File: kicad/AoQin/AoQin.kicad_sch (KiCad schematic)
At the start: 12 parts, among them J1 Conn_02x03_Odd_Even, J10 1869237, J3 1869237, J4 1869237, J5 1869237, J6 1869237, J7 1869237, J8 Screw_Terminal_01x03, J9 Screw_Terminal_01x03

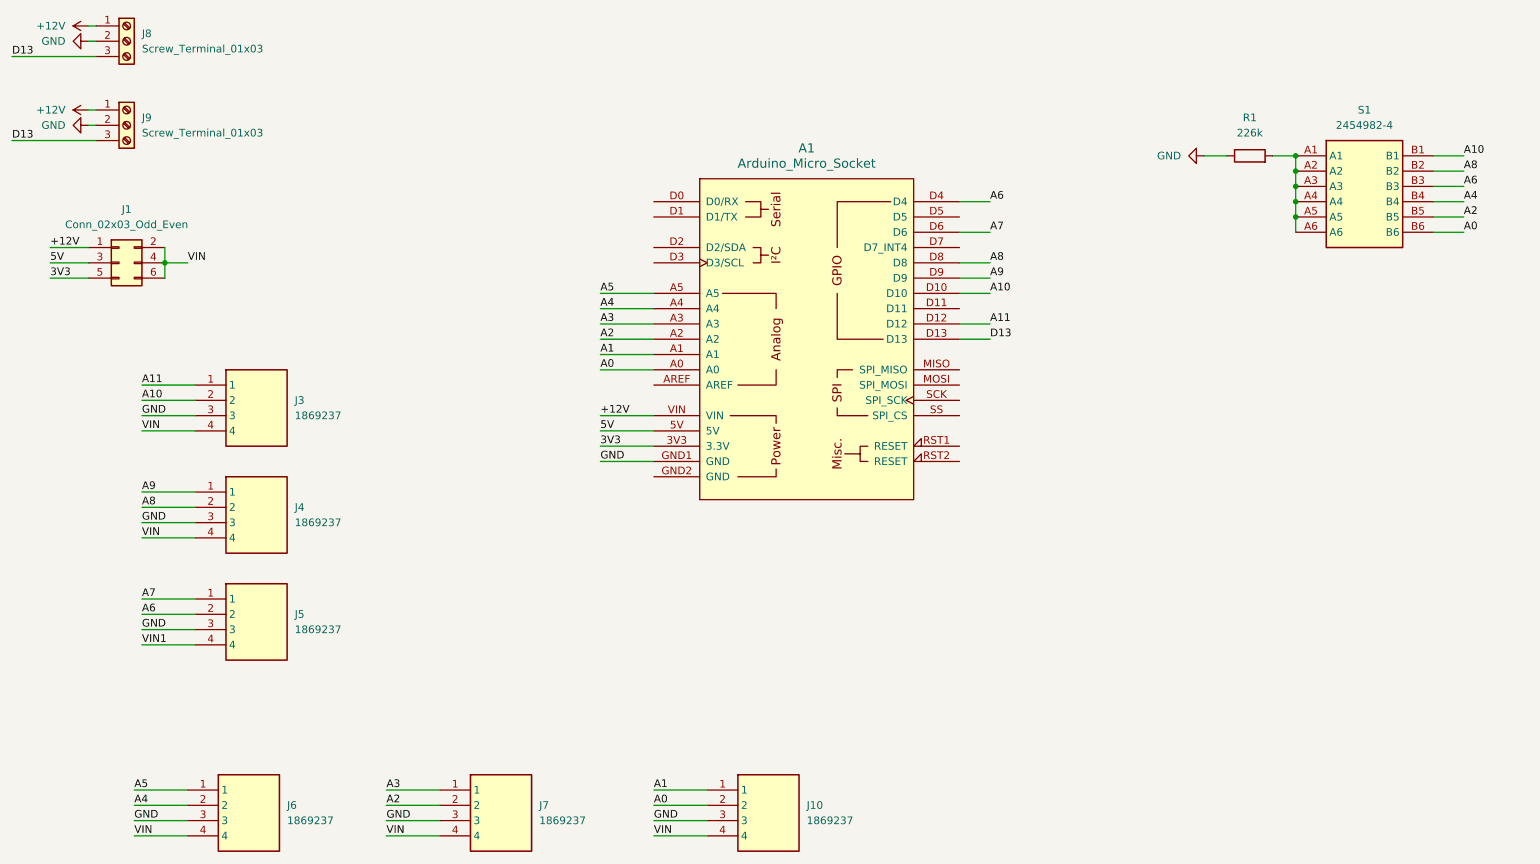
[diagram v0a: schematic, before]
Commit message: If I Had a Hammer
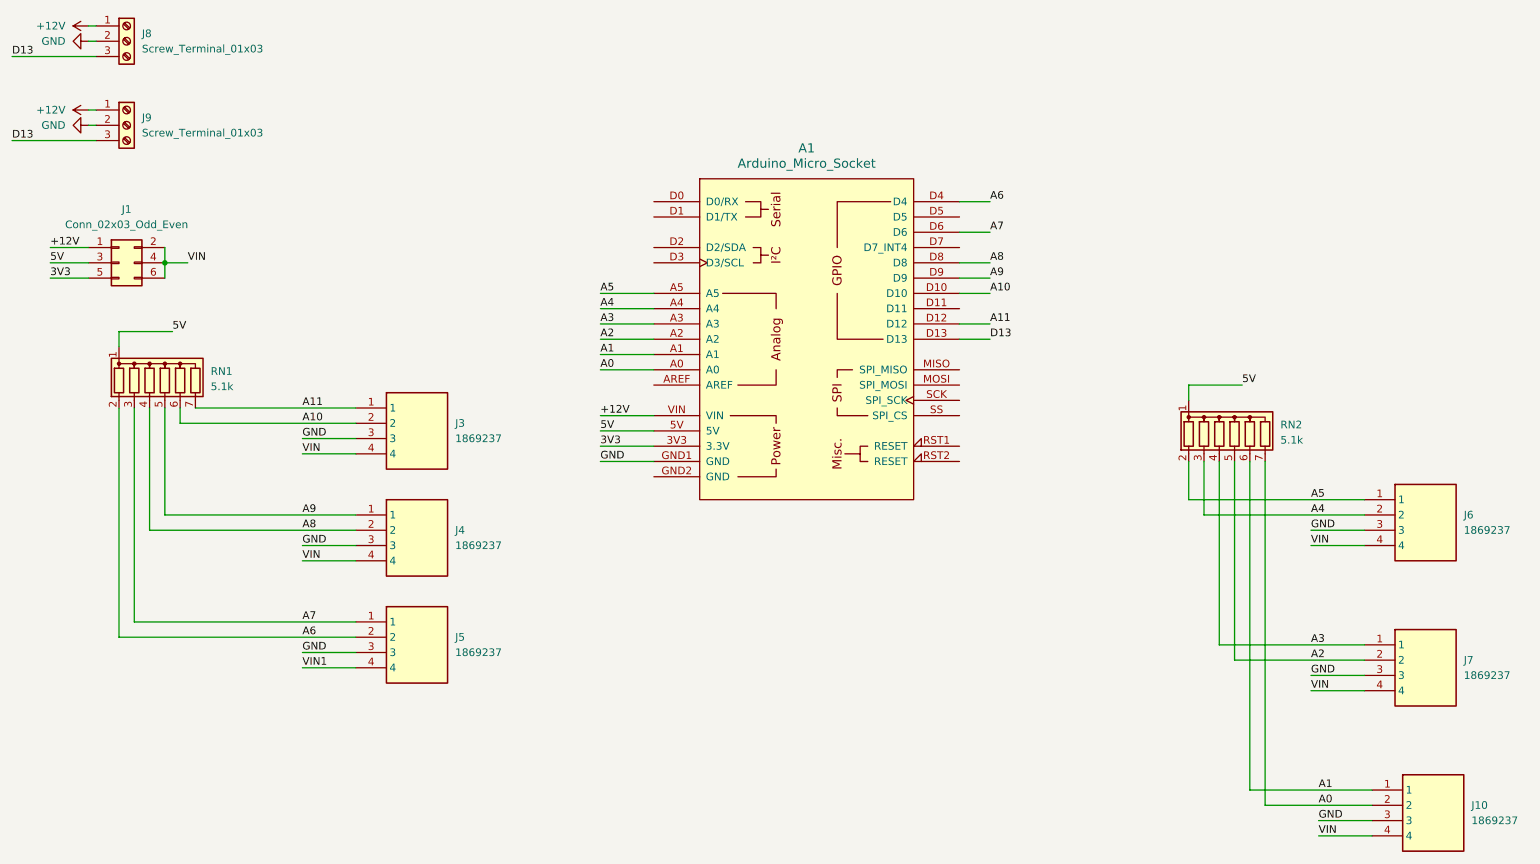
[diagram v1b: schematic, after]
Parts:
- removed R1: 226k, Resistor_THT:R_Axial_DIN0207_L6.3mm_D2.5mm_P7.62mm_Horizontal, symbol Device:R
- removed S1: 2454982-4, footprints:24549824, symbol 2454982-4:2454982-4
- added RN1, RN2: 5.1k, Resistor_THT:R_Array_SIP7, symbol Device:R_Network06
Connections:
- net 5V: now also RN1.1 (common), RN2.1 (common)
- net A0: now also RN2.7 (R6)
- net A1: now also RN2.6 (R5)
- net A10: now also RN1.6 (R5)
- net A11: now also RN1.7 (R6)
- net A2: now also RN2.5 (R4)
- net A3: now also RN2.4 (R3)
- net A4: now also RN2.3 (R2)
- net A5: now also RN2.2 (R1)
- net A6: now also RN1.2 (R1)
- net A7: now also RN1.3 (R2)
- net A8: now also RN1.4 (R3)
- net A9: now also RN1.5 (R4)
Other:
- moved on the sheet: J10, J3, J4, J5, J6, J7
